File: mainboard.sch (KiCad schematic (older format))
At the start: 73 parts, among them J1 Conn_01x06, J2 10118194-0001LF, J3 Micro_SD_Card, J4 xf2m-2415-1a, J5 XF2M-1015-1A, J6 U.FL-R-SMT-1, J7 U.FL-R-SMT-1, J9 Conn_01x02, Q1 RADFET, SW1 KMR231NG LFS, U1 RFM95W-915S2, U10 TPS22918-Q1, U11 DRV8830DRC, U2 ATSAMD51G_TQFN48, U3 DRV8830DRC, U4 TPS82740BSIPR, U5 DRV8830DRC, U6 MAX708RESA-T, U7 BMX160, U8 RFM95W-915S2, U9 ADS124S06IRHBR

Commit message: schematic work
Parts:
- removed C2: 10uF, Capacitor_SMD:C_0402_1005Metric, symbol mainboard-rescue:C_Small-Device
- removed C5: 1uF, Capacitor_SMD:C_0402_1005Metric, symbol mainboard-rescue:C_Small-Device
- removed J6, J7: U.FL-R-SMT-1, custom-footprints:U.FL-R-SMT-1, symbol mainboard-rescue:U.FL-R-SMT-1-symbols
- removed L1: 10uH, Inductor_SMD:L_0805_2012Metric, symbol mainboard-rescue:L_Small-Device
- removed R16, R17: 10K, Resistor_SMD:R_0402_1005Metric, symbol mainboard-rescue:R_US-Device
- removed U1, U8: RFM95W-915S2, RF_Module:HOPERF_RFM9XW_SMD, symbol mainboard-rescue:RFM95W-915S2-RF_AM_FM
- removed U2: ATSAMD51G_TQFN48, ATSAMD51G19A-MU:QFN50P700X700X90-49N-D, symbol mainboard-rescue:ATSAMD51G_TQFN48-
- added C?: 10uF, Capacitor_SMD:C_0402_1005Metric, symbol mainboard-rescue:C_Small-Device
- added C?: 1uF, Capacitor_SMD:C_0402_1005Metric, symbol mainboard-rescue:C_Small-Device
- added C? (x2): 0.1uF, Capacitor_SMD:C_0402_1005Metric, symbol mainboard-rescue:C_Small-Device
- added J?: U.FL-R-SMT-1, custom-footprints:U.FL-R-SMT-1, symbol mainboard-rescue:U.FL-R-SMT-1-symbols
- added L?: 10uH, Inductor_SMD:L_0805_2012Metric, symbol mainboard-rescue:L_Small-Device
- added R? (x2): 10K, Resistor_SMD:R_0402_1005Metric, symbol mainboard-rescue:R_US-Device
- added U?: RFM98PW-symbols, custom-footprints:RFM95PW, symbol mainboard-rescue:RFM98PW-symbols
- added U?: ATSAMD51J20A-M, Package_DFN_QFN:QFN-64-1EP_9x9mm_P0.5mm_EP4.7x4.7mm, symbol MCU_Microchip_SAMD:ATSAMD51J20A-M
- U10: symbol wbraun_ic_lib:TPS22918-Q1 -> mainboard-rescue:TPS22918-Q1-wbraun_ic_lib
- U11, U3, U5: symbol wbraun_ic_lib:DRV8830DRC -> mainboard-rescue:DRV8830DRC-wbraun_ic_lib
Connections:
- net +3V3: now also R5.2, C?.1, R?.2, U?.21 (VDDIOB), U?.34 (VDDIO), U?.48 (VDDIO), U?.56 (VDDIO), U?.8 (VDDANA), U?.9 (3.3V); no longer R5.1
- net ADC_CS: now also U?.40 (PB17)
- net BATTERY: now also C?.1, U?.15 (PA06)
- net BATT_P: now also U?.5 (VCC)
- net BURN1: now also U?.59 (PB30)
- net BURN2: now also U?.60 (PB31)
- net CS_CAM: now also U?.28 (PB15)
- net CS_SD: now also U?.51 (PA27)
- net EN_CAM: now also U?.39 (PB16)
- net GND: now also C?.2, C?.2, C?.2, C?.2, J?.1 (GND), J?.2, R?.1, U?.16 (GND), U?.17 (GND), U?.2 (GND), U?.22 (GND), U?.33 (GND), U?.47 (GND), U?.54 (GND), U?.65 (GND), U?.7 (GNDANA)
- net MISO: now also U?.10 (MISO), U?.31 (PA14)
- net MOSI: now also U?.11 (MOSI), U?.29 (PA12)
- net RF2_CS: now also R?.1, U?.13 (NSS)
- net SCK: now also U?.12 (SCK), U?.30 (PA13)
- net SCL1: now also U?.26 (PB13)
- net SCL2: now also R7.1, U?.35 (PA16); no longer R8.1
- net SDA1: now also U?.25 (PB12)
- net SDA2: now also R8.1, U?.36 (PA17); no longer R7.1
- net SWCLK: now also R5.1, U?.57 (PA30); no longer R5.2
- net SWDIO: now also U?.58 (PA31)
- net WDT_WDI: now also R?.2, U?.44 (PA23)
- net ~RESET: now also U?.52 (~RESET)
- net at D3.4 (DIN): now also U?.42 (PA21)
- net USB+ renamed USB_D+
- net USB_D+: now also U?.46 (PA25)
- net USB- renamed USB_D-
- net USB_D-: now also U?.45 (PA24)
- new net: J?.3 (ANT), U?.1 (ANT)
- new net: C?.1, C?.1, L?.2, U?.53 (VDDCORE)
- new net: L?.1, U?.55 (VSW)
- new net RF_BUSY: U?.14 (PA05), U?.4 (GPIO_4)
- new net RF_CS: U?.12 (PB09)
- new net RF_IO1: U?.13 (PA04), U?.7 (GPIO_1)
- new net RF_IO2: U?.8 (GPIO_2)
- new net RF_RST: U?.14 (RESET), U?.27 (PB14)
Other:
- note removed: "I2C_1\nSCL: PA01\nSDA: PA00\n\nI2C_2\nSCL: PA16\nSDA: PA17\n"
- note removed: "LoRa RADIO\n"
- moved on the sheet: C1, C15, C3, C6, C7, D3, J1, J2, R10, R2, R4, R5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

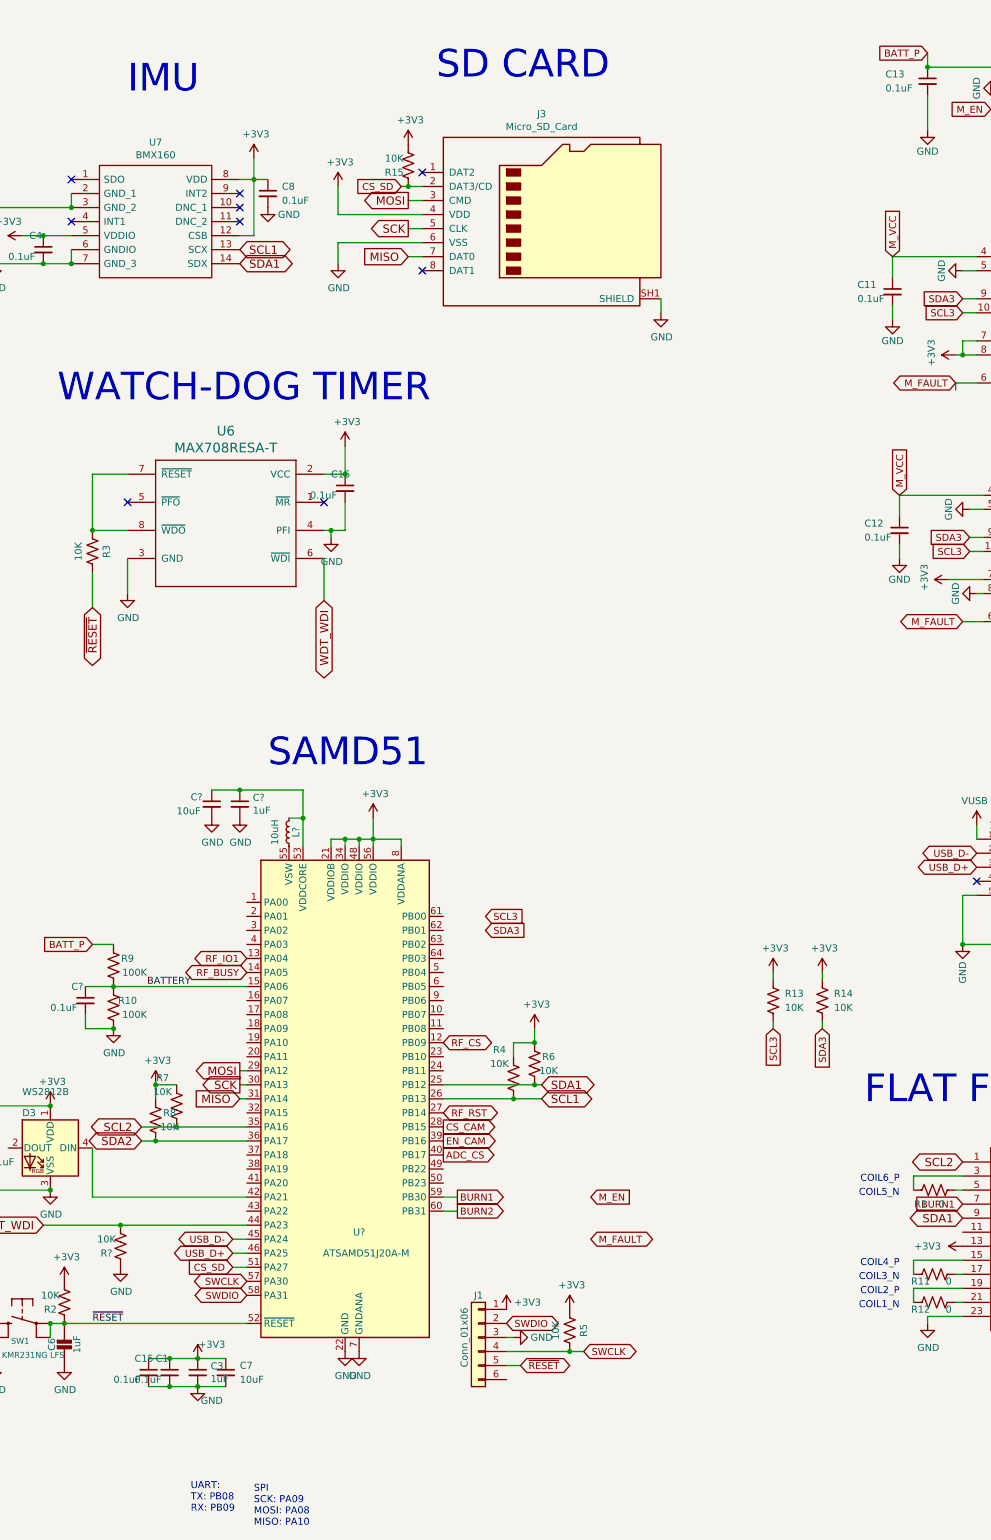
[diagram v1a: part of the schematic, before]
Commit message: finished schematic changes
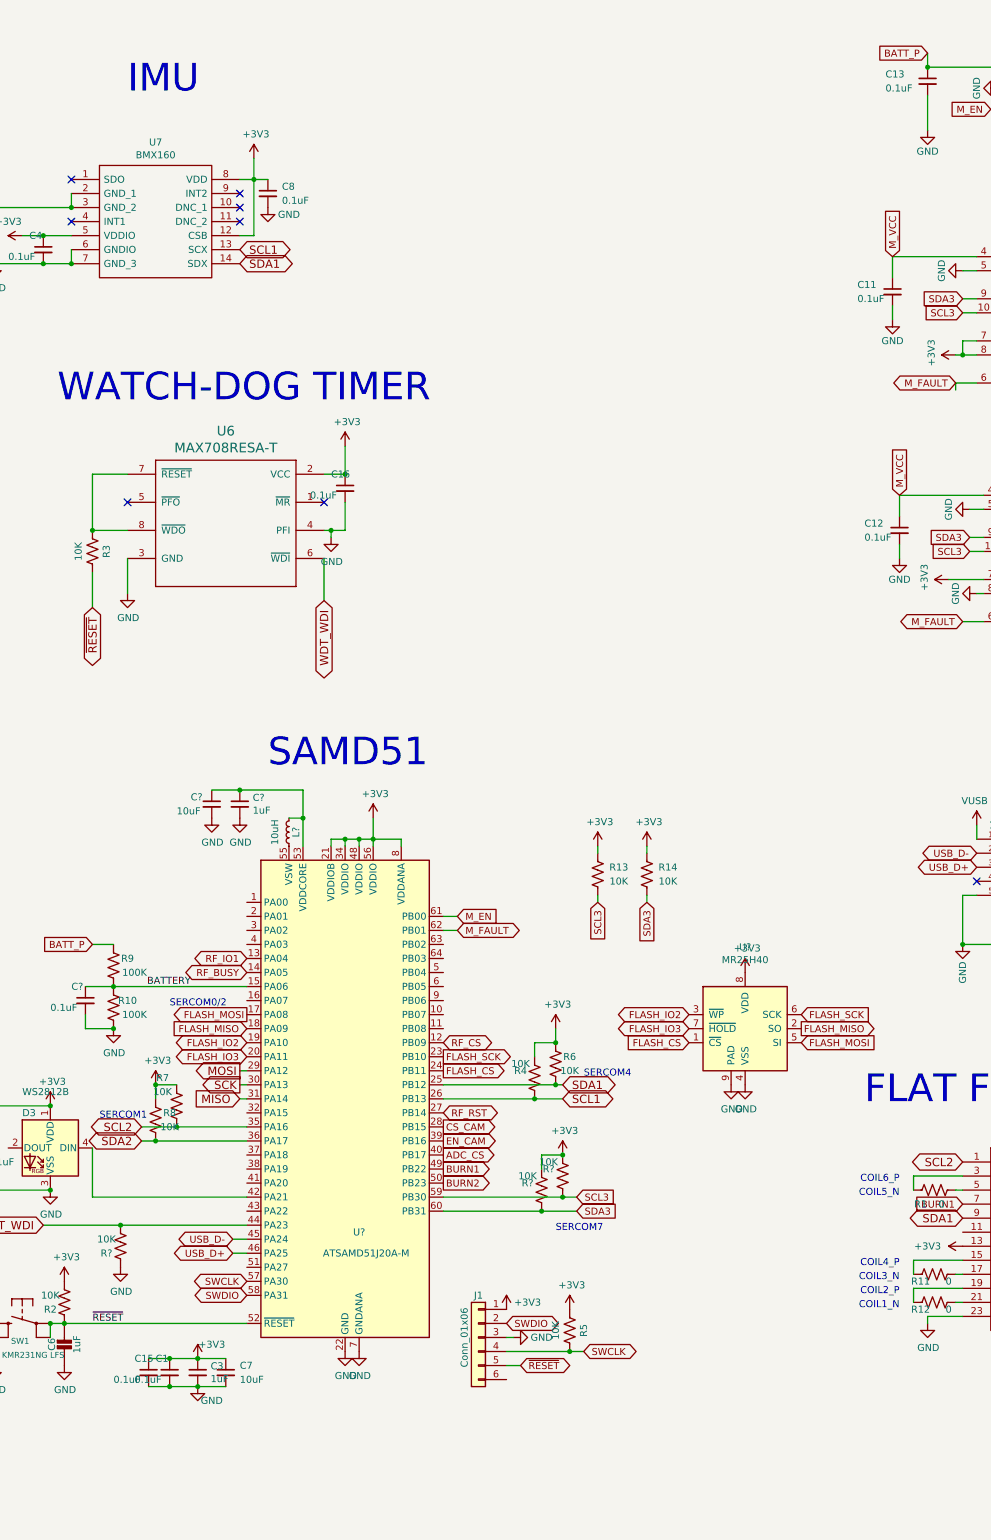
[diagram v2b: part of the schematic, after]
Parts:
- removed J3: Micro_SD_Card, custom-footprints:503182-1853_MOLEX-MicroSD, symbol mainboard-rescue:Micro_SD_Card-Connector
- removed R15: 10K, Resistor_SMD:R_0402_1005Metric, symbol mainboard-rescue:R_US-Device
- added R? (x2): 10K, Resistor_SMD:R_0402_1005Metric, symbol mainboard-rescue:R_US-Device
- added U?: MR25H40, symbol Memory_NVRAM:MR25H40
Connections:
- net +3V3: now also R?.2, R?.2, U?.8 (VDD)
- net BURN1: now also U?.49 (PB22); no longer U?.59 (PB30)
- net BURN2: now also U?.50 (PB23); no longer U?.60 (PB31)
- net GND: now also U?.4 (VSS), U?.9 (PAD)
- net M_EN: now also U?.61 (PB00)
- net M_FAULT: now also U?.62 (PB01)
- net SCL3: now also U?.59 (PB30), R?.1
- net SDA3: now also U?.60 (PB31), R?.1
- net FLASH_MOSI: now reaches U?.17 (PA08)
- net FLASH_MOSI: now also U?.5 (SI)
- net FLASH_MISO: now reaches U?.18 (PA09)
- net FLASH_MISO: now also U?.2 (SO)
- net FLASH_IO2: now reaches U?.19 (PA10)
- net FLASH_IO2: now also U?.3 (~WP)
- net FLASH_IO3: now reaches U?.20 (PA11)
- net FLASH_IO3: now also U?.7 (~HOLD)
- net FLASH_SCK: now reaches U?.23 (PB10)
- net FLASH_SCK: now also U?.6 (SCK)
- net FLASH_CS: now reaches U?.24 (PB11)
- net FLASH_CS: now also U?.1 (~CS)
- net CS_SD: no longer names the net of U?.51 (PA27)
- no-connect marks 12 -> 10
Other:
- note added: "SERCOM0/2"
- note added: "SERCOM1"
- note added: "SERCOM4\n"
- note added: "SERCOM7"
- note removed: "SD CARD"
- note removed: "SPI\nSCK: PA09\nMOSI: PA08\nMISO: PA10\n"
- note removed: "UART:\nTX: PB08\nRX: PB09\n"
- moved on the sheet: R13, R14, R4, R6
